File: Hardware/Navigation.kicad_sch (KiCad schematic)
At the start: 54 parts, among them J1 USB_C_Receptacle_USB2.0_16P, J2 SM03B-SRSS-TB_LF__SN_, Q3 2N7002, U1 RP2350B, U11 W25Q128JVS, U20 TLV75733PDRV, U3 TPS2113ADRBR, Y1 ABM8-272-T3

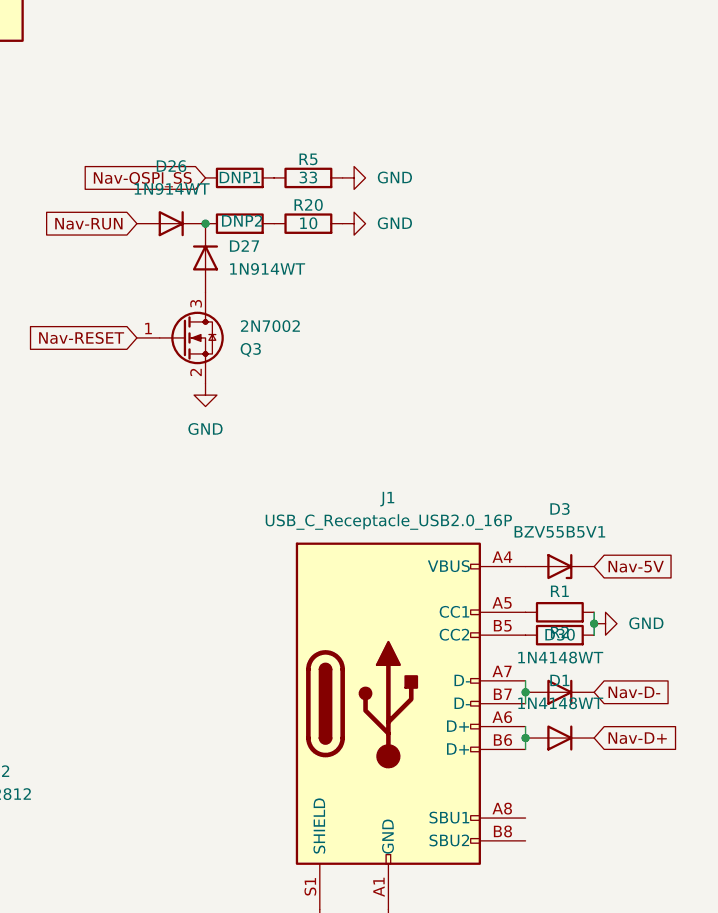
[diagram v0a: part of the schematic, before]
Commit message: test gpg
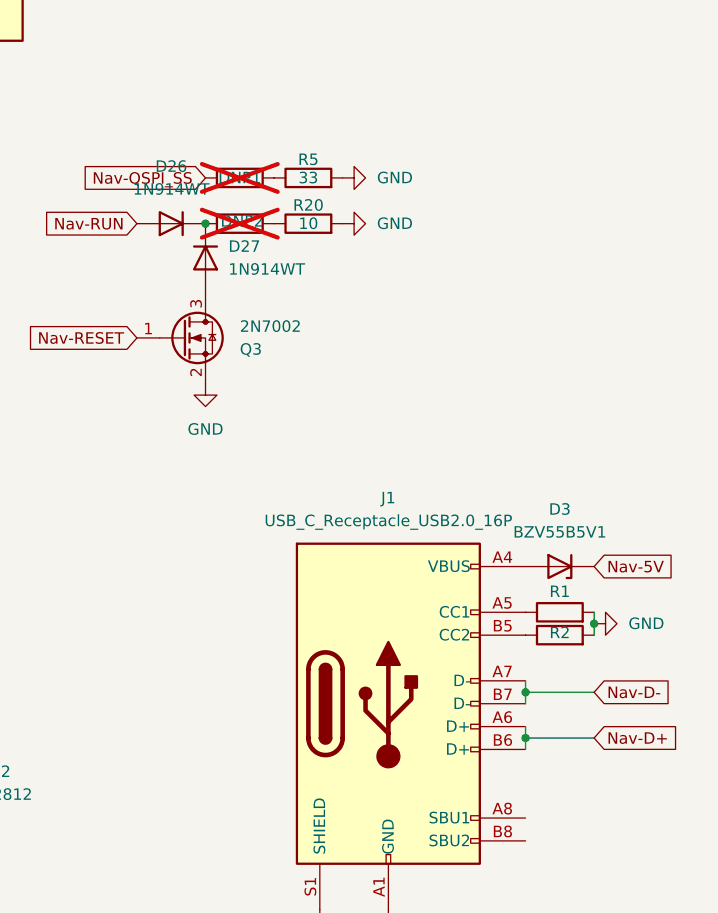
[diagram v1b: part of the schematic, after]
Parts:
- removed D1, D30: 1N4148WT, Diode_SMD:D_SOD-523, symbol Diode:1N4148WT
- DNP1, DNP2: now not fitted
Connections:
- net Nav-D+: now also J1.A6 (D+), J1.B6 (D+)
- net Nav-D-: now also J1.A7 (D-), J1.B7 (D-)
